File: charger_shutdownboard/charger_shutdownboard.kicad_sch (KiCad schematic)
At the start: 30 parts, among them J1 Acc SFC, J2 12V Power supply, J3 CAN COTS Charger, J4 Shutdown Button, J5 Reset Button, J6 TSMP to HV, J7 TSMP to Banana Jacks, J8 J1772 Negotiation, U1 NUCLEO-L432KC, U3 ISO1050DUB, U4 LM7809_TO220

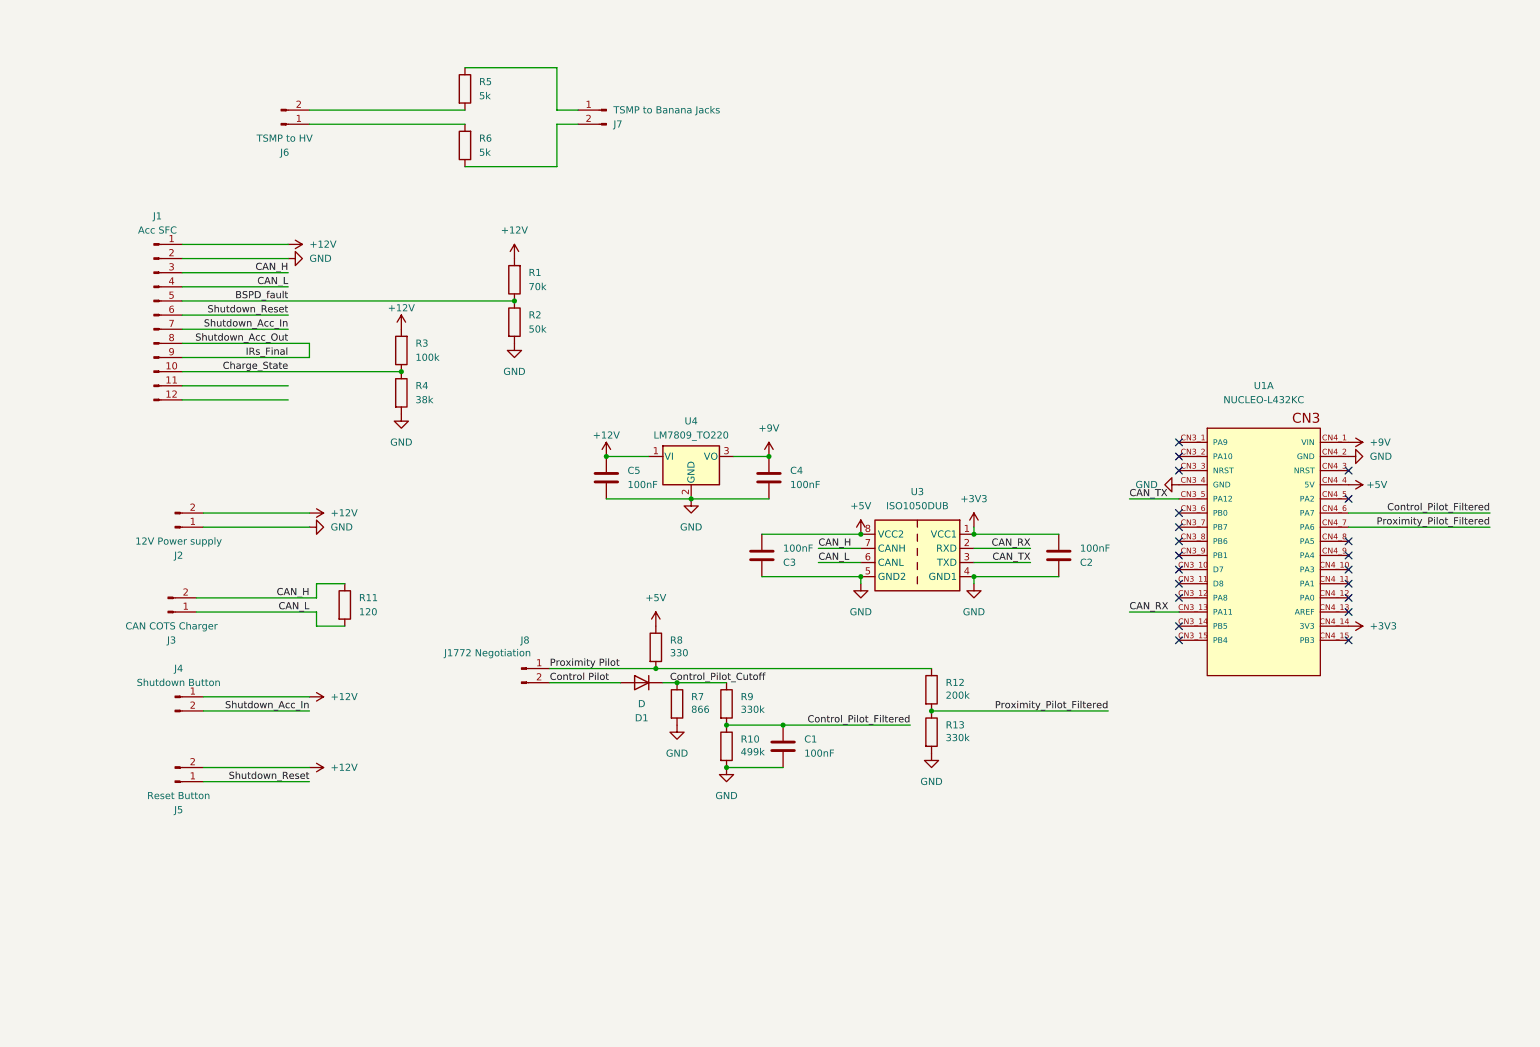
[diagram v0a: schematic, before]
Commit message: Revised PCB for J1772 negotiation
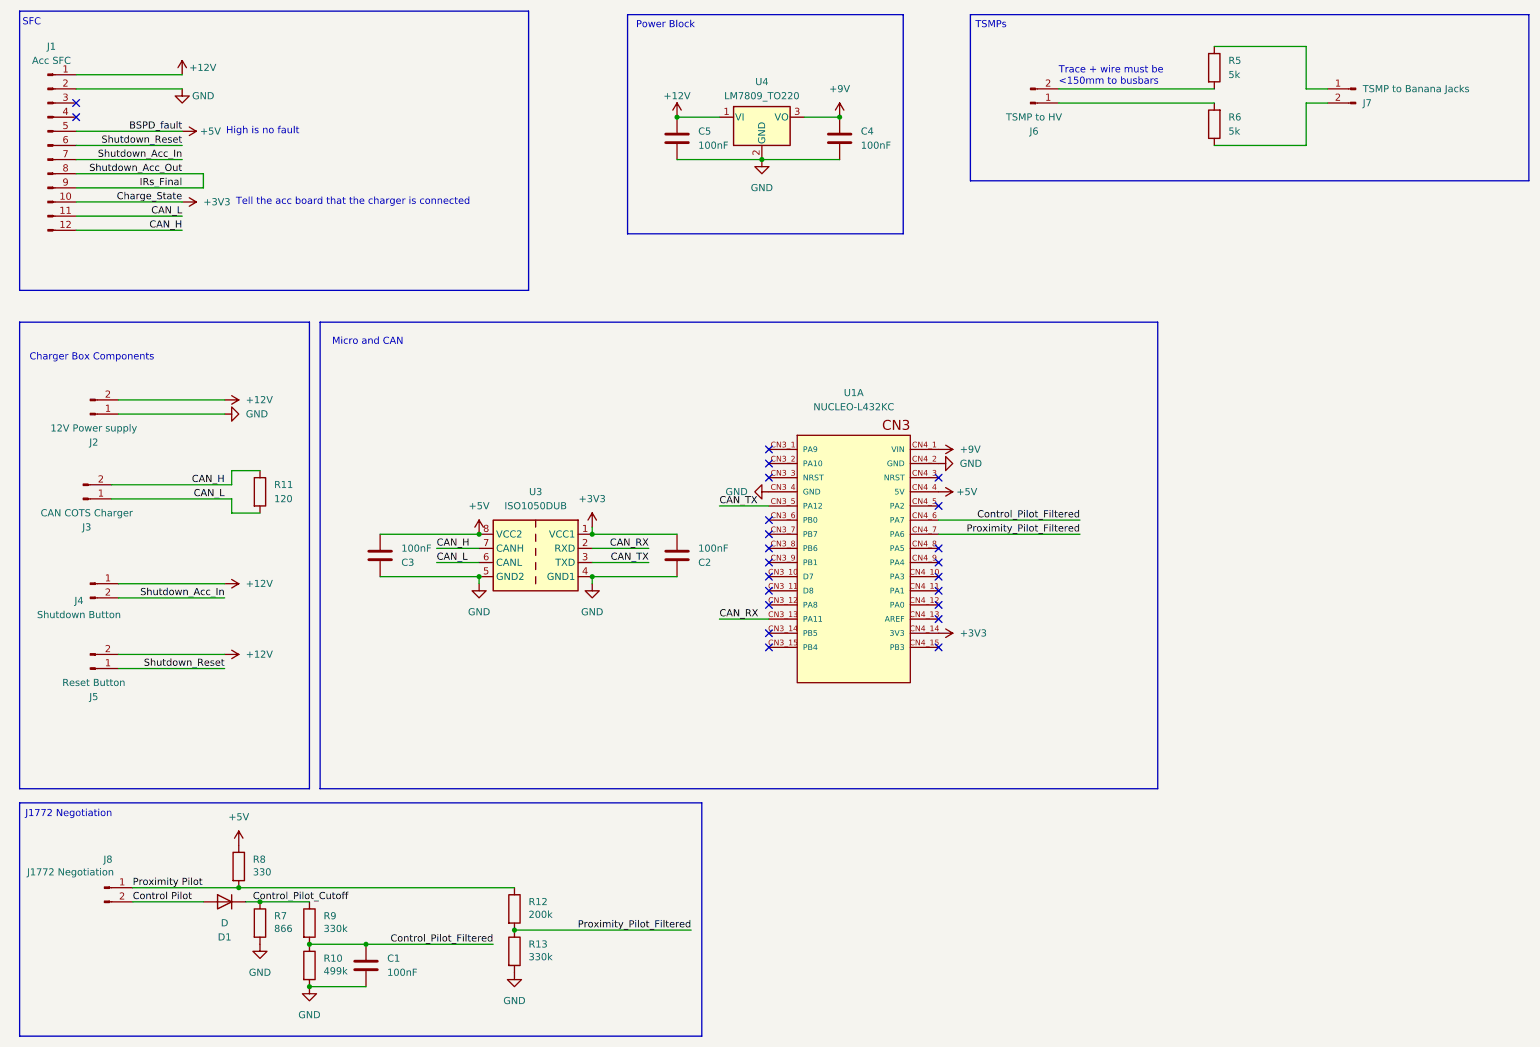
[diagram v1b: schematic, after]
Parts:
- removed R1: 70k, Resistor_SMD:R_0805_2012Metric_Pad1.20x1.40mm_HandSolder, symbol Device:R
- removed R2: 50k, Resistor_SMD:R_0805_2012Metric_Pad1.20x1.40mm_HandSolder, symbol Device:R
- removed R3: 100k, Resistor_SMD:R_0805_2012Metric_Pad1.20x1.40mm_HandSolder, symbol Device:R
- removed R4: 38k, Resistor_SMD:R_0805_2012Metric_Pad1.20x1.40mm_HandSolder, symbol Device:R
- C1, C2, C3, C4, C5: footprint (none) -> Capacitor_SMD:C_0805_2012Metric_Pad1.18x1.45mm_HandSolder
- D1: footprint (none) -> Diode_SMD:D_0805_2012Metric_Pad1.15x1.40mm_HandSolder
- R10, R12, R13, R7, R8, R9: footprint (none) -> Resistor_SMD:R_0805_2012Metric_Pad1.20x1.40mm_HandSolder
- U1: footprint NUCLEO-L432KC:MODULE_NUCLEO-L432KC -> FS_3_Global_Footprint_Library:NUCLEO-L432KC
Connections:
- net BSPD_fault is gone; now on net +5V: J1.5 (Pin_5)
- net Charge_State is gone; now on net +3V3: J1.10 (Pin_10)
- net CAN_H: now also J1.12 (Pin_12); no longer J1.3 (Pin_3)
- net CAN_L: now also J1.11 (Pin_11); no longer J1.4 (Pin_4)
- no-connect marks 21 -> 23
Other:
- note added: "Charger Box Components"
- note added: "High is no fault"
- note added: "J1772 Negotiation"
- note added: "Micro and CAN"
- note added: "Power Block"
- note added: "SFC"
- note added: "TSMPs"
- note added: "Tell the acc board that the charger is connected"
- note added: "Trace + wire must be <150mm to busbars"
- moved on the sheet: C1, C2, C3, C4, C5, D1, J1, J2, J3, J4, J5, J6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
